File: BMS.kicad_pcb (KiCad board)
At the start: 2 copper layers, 78 parts, among them J1 Screw_Terminal_01x02, J5 BATT_PACK -, J6 PACK _PACK -, Q22 CSD19531Q5A, Q23 CSD19531Q5A, Q24 CSD19531Q5A, T3 EE20_10_6_750811647, U1 TL431DBZ, U18 VIPer26LD, U2 PC817, U21 BQ7790500PWR, U3 LM3914N

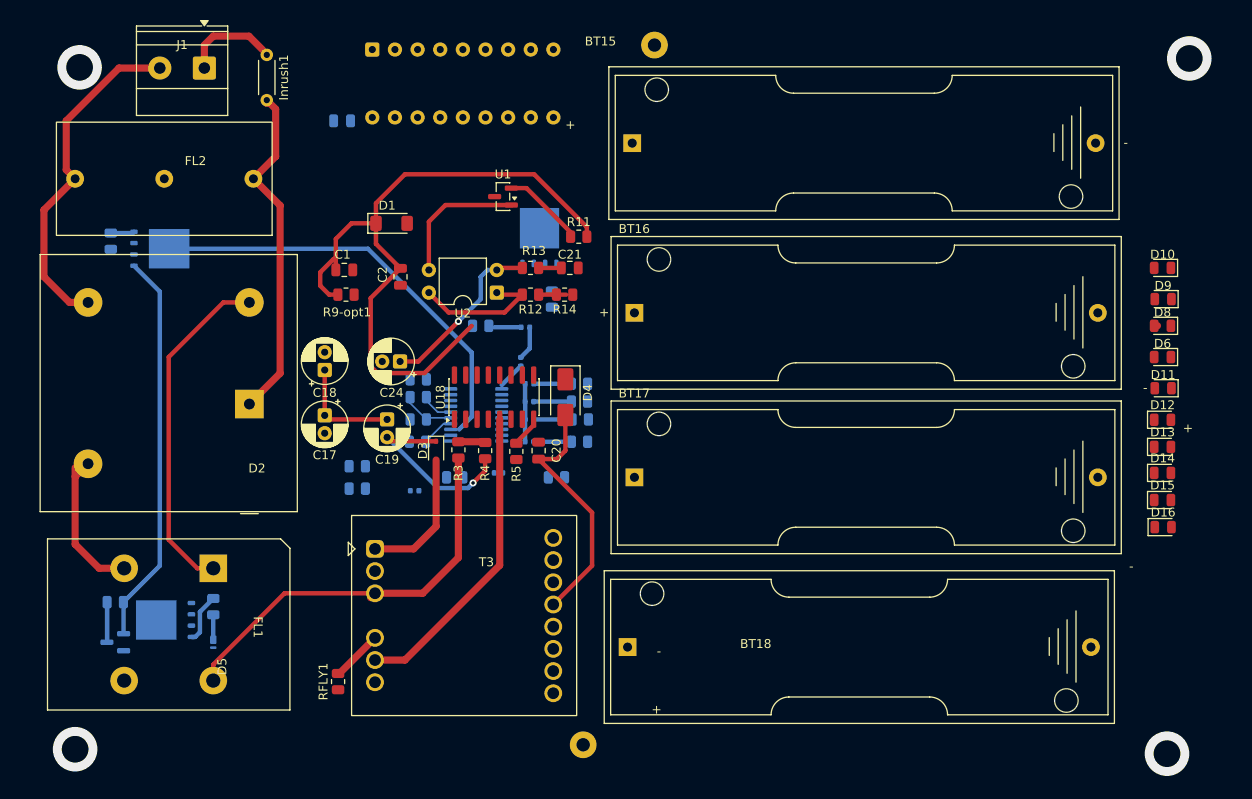
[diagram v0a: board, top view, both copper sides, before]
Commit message: Routing update
 19 errors to go
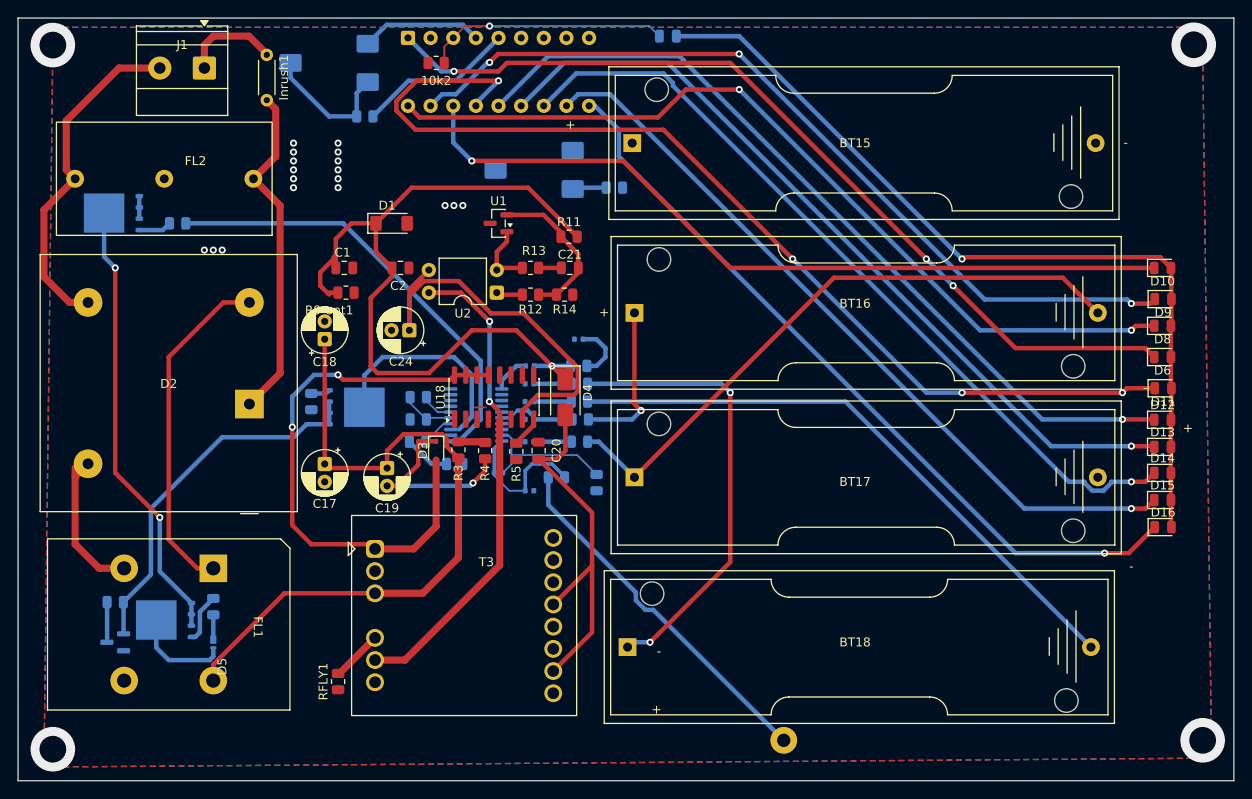
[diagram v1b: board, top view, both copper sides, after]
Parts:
- removed J6: PACK _PACK -, TerminalBlock_MetzConnect:TerminalBlock_MetzConnect_360271_1x01_Horizontal_ScrewM3.0_Boxed
- added RV1: R_Pot_Trim, Resistor_SMD:R_0805_2012Metric, B.Cu at (134.0, 51.0)
- added RV2: R_Pot_Trim, Potentiometer_SMD:Potentiometer_ACP_CA6-VSMD_Vertical, B.Cu at (153.0, 57.0)
- added RV3: R_Pot_Trim, Potentiometer_SMD:Potentiometer_ACP_CA6-VSMD_Vertical, B.Cu at (130.0, 45.0)
- 10k2: moved to F.Cu
- moved J5 79.3 mm to (181.0, 121.0)
- moved Q22 47.9 mm to (105.8, 61.9), turned to 180 degrees
- moved 10k2 46.1 mm to (142.0, 45.0), turned to 0 degrees
- moved 10k3 44.4 mm to (162.0, 59.0)
- moved R1 42.9 mm to (113.0, 63.0), turned to 180 degrees
- moved C3 37.8 mm to (168.0, 42.0)
- moved R6 28.8 mm to (128.0, 83.0)
- moved Q23 28.2 mm to (132.9, 83.6)
- moved Rsrp1 23.1 mm to (160.0, 92.1), turned to -90 degrees
- moved C37 12.9 mm to (152.5, 93.0)
- moved RVO1 11.9 mm to (158.0, 79.0)
- moved C30 6.13 mm to (158.0, 76.0), turned to 0 degrees
- moved C17 5.46 mm to (129.5, 90.0)
- moved C19 5.46 mm to (136.5, 90.5)
- moved U3 4.21 mm to (138.8, 42.2)
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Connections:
- U2 pad 1: VDD_U18 -> Net-(R12-Pad2)
- U2 pad 2: FB -> Net-(U1-K)
- U2 pad 3: Net-(U1-K) -> FB
- U2 pad 4: Net-(R12-Pad2) -> VDD_U18
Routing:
- net Net-(D11-K): track 0.00 -> 115.7 mm, vias 0 -> 4
- net Net-(D6-K): track 0.00 -> 99.3 mm, vias 0 -> 3
- net Net-(D8-K): track 0.00 -> 97.0 mm, vias 0 -> 2
- net Net-(D9-K): track 0.00 -> 95.5 mm, vias 0 -> 3
- net Net-(D10-A): track 0.38 -> 95.6 mm, vias 0 -> 1
- net Net-(D12-K): track 0.00 -> 92.8 mm, vias 0 -> 1
- net Net-(D13-K): track 0.00 -> 90.9 mm, vias 0 -> 1
- net Net-(D14-K): track 0.00 -> 90.5 mm, vias 0 -> 1
- net Net-(D10-K): track 0.00 -> 88.8 mm, vias 0 -> 1
- net Net-(D16-K): track 0.00 -> 87.2 mm, vias 0 -> 1
- net Net-(D15-K): track 0.00 -> 86.1 mm, vias 0 -> 1
- net V+: track 0.00 -> 78.3 mm, vias 0 -> 3
- net PACK-: track 0.00 -> 72.6 mm
- net Net-(BT16--): track 0.00 -> 69.8 mm
- net Net-(BT15-+): track 0.00 -> 67.9 mm
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- added copper zone on B.Cu, net GND
- added copper zone on F.Cu, net GND
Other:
- board outline added: 136.4 x 85.6 mm
